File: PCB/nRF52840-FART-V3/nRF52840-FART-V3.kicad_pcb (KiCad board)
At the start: 2 copper layers, 44.4 x 22 mm, 7 parts, among them U1 xiao-ble

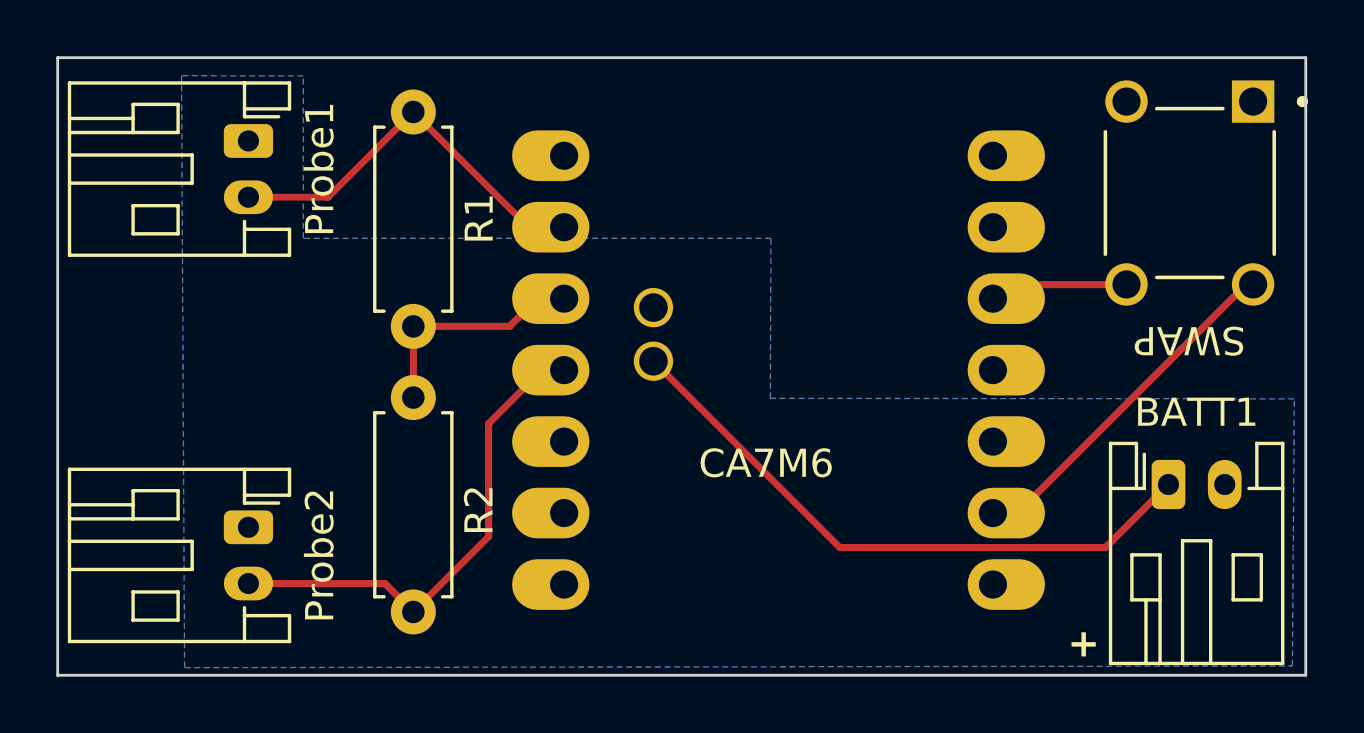
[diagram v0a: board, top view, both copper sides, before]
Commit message: Tweaks to the PCB design
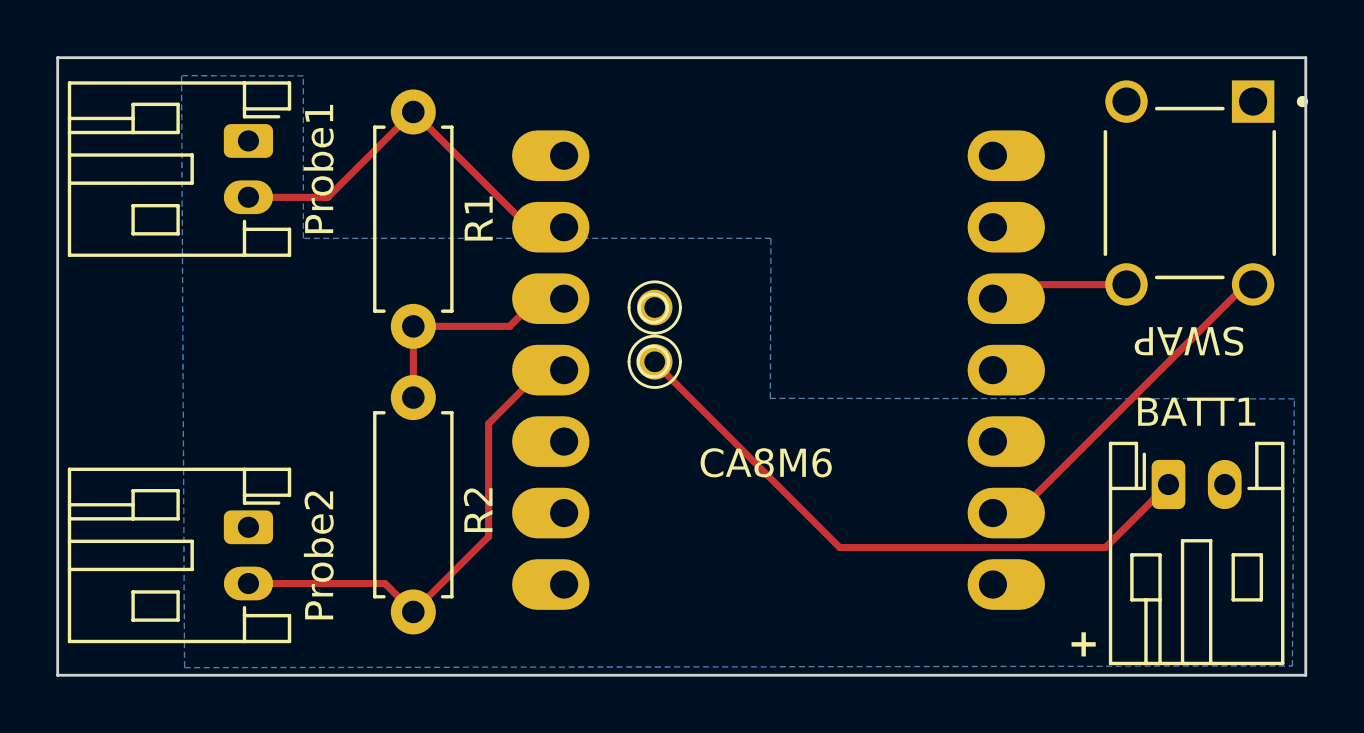
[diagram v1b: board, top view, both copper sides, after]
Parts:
- added J1: 0914-3-15-20-77-14-11-0, Samac:0914315207714110, F.Cu at (75.1, 57.9)
- added J2: 0914-3-15-20-77-14-11-0, Samac:0914315207714110, F.Cu at (75.1, 59.8)
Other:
- board text added: "CA8M6"
- board text removed: "CA7M6"
